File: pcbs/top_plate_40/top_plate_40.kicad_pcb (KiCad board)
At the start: 2 copper layers, 131.3 x 108 mm, 6 parts

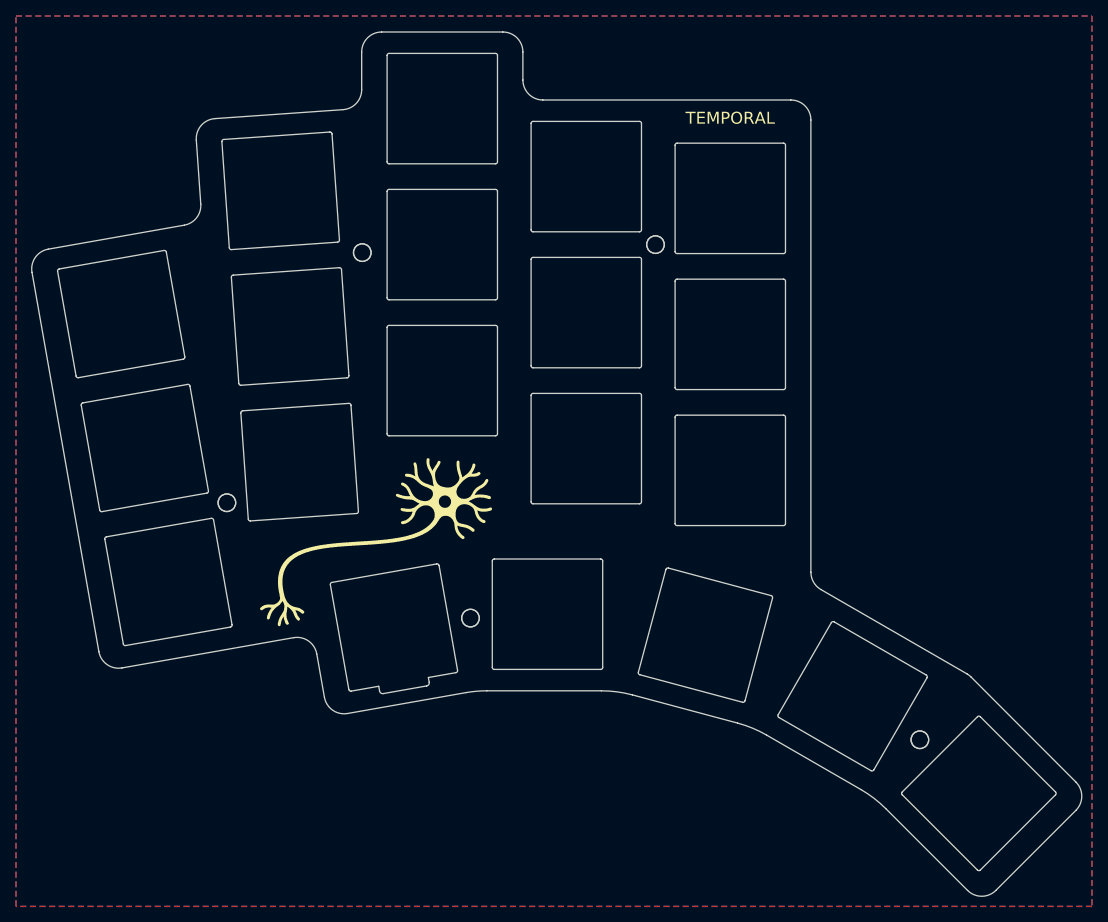
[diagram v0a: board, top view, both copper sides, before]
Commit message: update naming and gen files
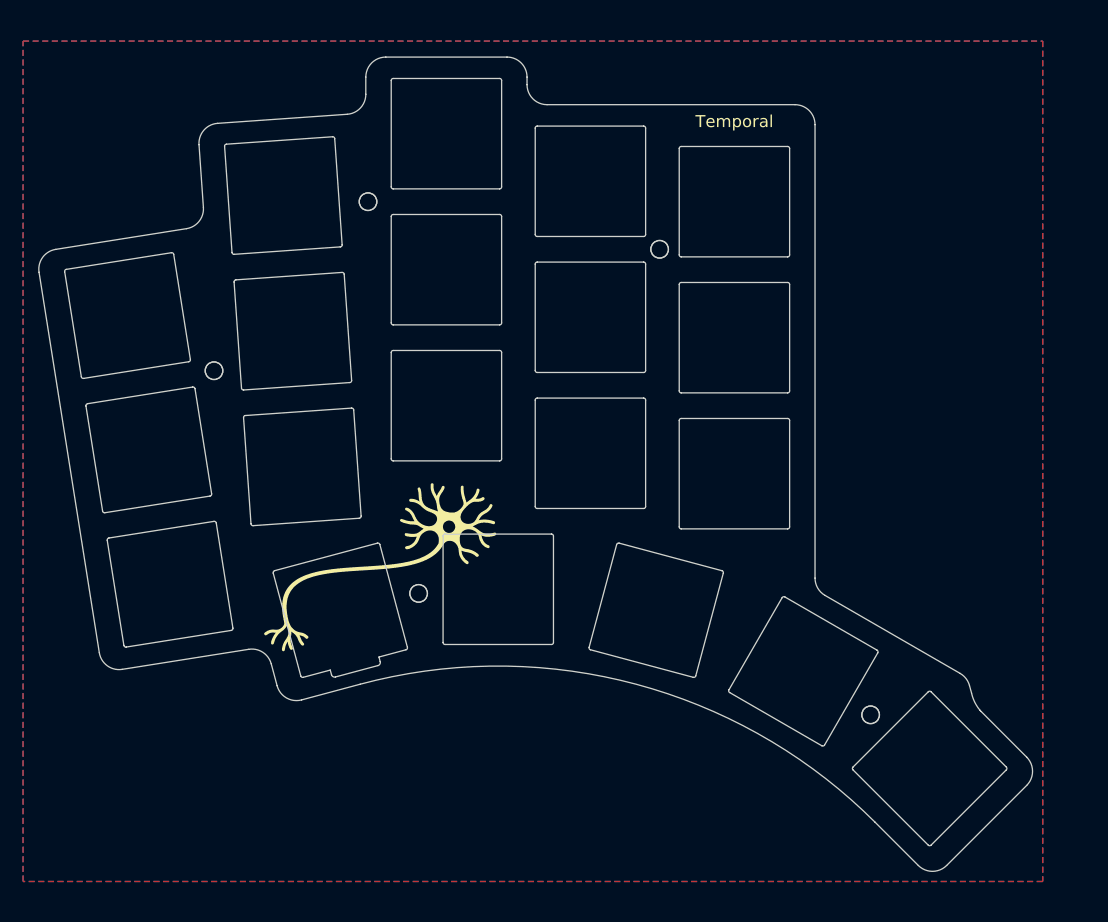
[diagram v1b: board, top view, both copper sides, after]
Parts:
- moved MH5 16.6 mm to (71.9, 61.8), turned to 9 degrees
- moved MH4 7.18 mm to (97.5, 89.6), turned to 15 degrees
- moved MH3 6.90 mm to (154.0, 104.8)
- moved MH1 6.41 mm to (91.1, 40.6)
- moved G1 3.18 mm to (92.7, 86.3)
- moved MH2 0.78 mm to (127.6, 46.6)
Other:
- board size 131.3 x 108 mm -> 124.2 x 101.8 mm
- board text added: "Temporal"
- board text removed: "TEMPORAL"
